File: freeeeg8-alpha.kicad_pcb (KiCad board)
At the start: 2 copper layers, 26 x 26 mm, 33 parts, among them J1 AIN0, J10 GND, J12 STACK_1, J13 STACK_2, J14 XIAO_1, J15 XIAO_2, J2 AIN1, J3 AIN2, J4 AIN3, J5 AIN4, J6 AIN5, J7 AIN6, J8 AIN7, J9 AINREF, U1 ADC, U2 AVDD, U3 DVDD, X1 XTAL

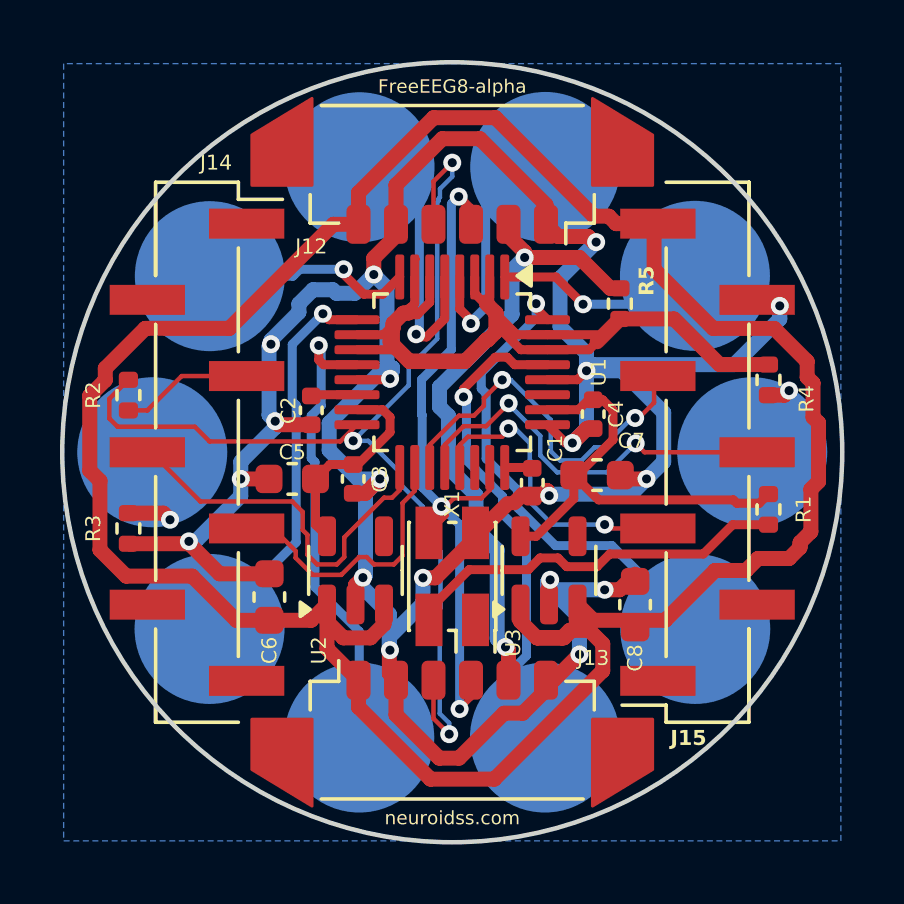
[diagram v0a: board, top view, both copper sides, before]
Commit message: Add files via upload
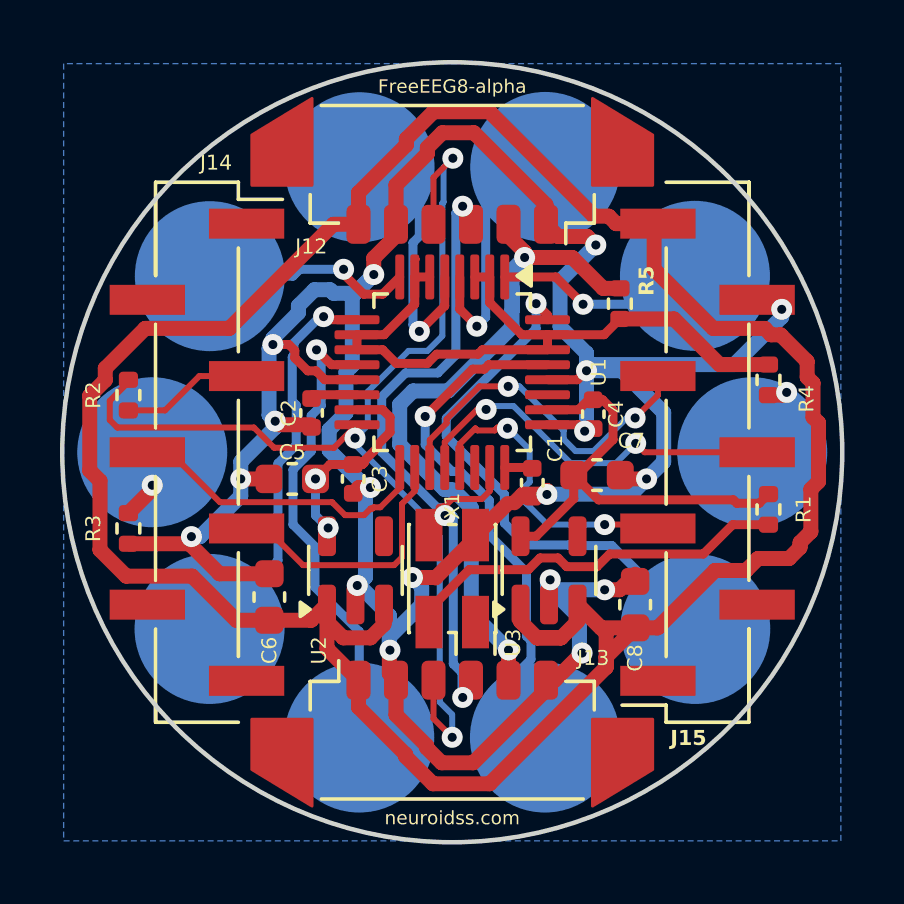
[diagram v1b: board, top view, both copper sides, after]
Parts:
- moved C2 0.09 mm to (-4.69, -1.31)
- moved X1 0.07 mm to (0.00, 4.21)
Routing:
- net /AINREF: track 37.8 -> 23.8 mm
- net /AINREF_STACK: track 21.3 -> 24.1 mm
- net /GND_POGOPIN: track 3.97 -> 1.26 mm
- net /CS: track 12.7 -> 10.3 mm
- net /5V: track 87.4 -> 89.8 mm
- net /AIN1P: track 16.4 -> 17.9 mm
- net /AIN0P: track 16.3 -> 17.7 mm
- net /SYNC/RESET_ADC: track 36.7 -> 38.1 mm
- net /GND: track 113.2 -> 112.3 mm, vias 19 -> 18
- net /SCLK: track 12.7 -> 11.8 mm
- net /DOUT: track 13.6 -> 12.9 mm
- net /XTAL1/CLKIN: track 28.4 -> 29.0 mm
- net /AVDD: track 7.08 -> 7.21 mm, vias 0 -> 2

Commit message: Add files via upload
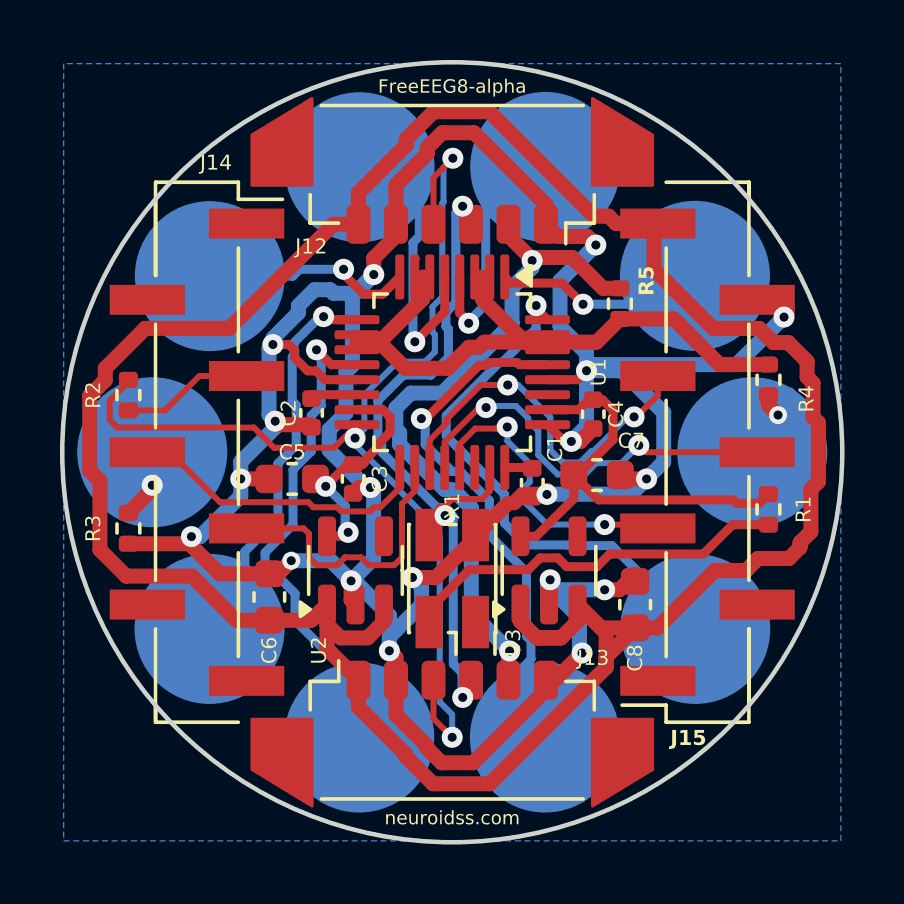
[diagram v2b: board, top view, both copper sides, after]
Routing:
- net /GND: track 112.3 -> 116.4 mm, vias 18 -> 19
- net /AINREF_POGOPIN: track 4.97 -> 2.49 mm
- net /AINREF: track 23.8 -> 24.8 mm
- net /SCLK: track 11.8 -> 12.6 mm
- net /DOUT: track 12.9 -> 13.7 mm
- net /AIN7P: track 15.8 -> 16.6 mm
- net /AINREF_STACK: track 24.1 -> 23.4 mm
- net /AIN4P: track 9.15 -> 9.84 mm
- net /DRDY: track 8.96 -> 9.64 mm
